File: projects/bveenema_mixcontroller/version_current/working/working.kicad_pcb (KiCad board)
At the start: 2 copper layers, 150.2 x 127 mm, 174 parts, among them J101 B2B-PH-K-S(LF)(SN), J103 B3B-PH-K-S(LF)(SN), J104 B2B-XH-A(LF)(SN), J11 B5B-XH-A(LF)(SN), J13 B8B-XH-A(LF)(SN), J2 B2B-XH-A(LF)(SN), J38 B5B-PH-K-S(LF)(SN), J67 B6B-PH-K-S(LF)(SN), J7 B3B-XH-A(LF)(SN), J9 B2B-XH-A(LF)(SN), J91 B4B-XH-A(LF)(SN), J94 0705430001, J95 B8B-XH-A(LF)(SN), J97 B4B-PH-K-S(LF)(SN), Q1 Q_NMOS_GDS, Q2 Q_NMOS_GDS, U1 Photon, U2 Adafruit_1096, U3 BOB-12009, U4 BOB-12009, U6 HSCDANN005PGAA5, U7 MCP23017_SP, U8 ADS7830

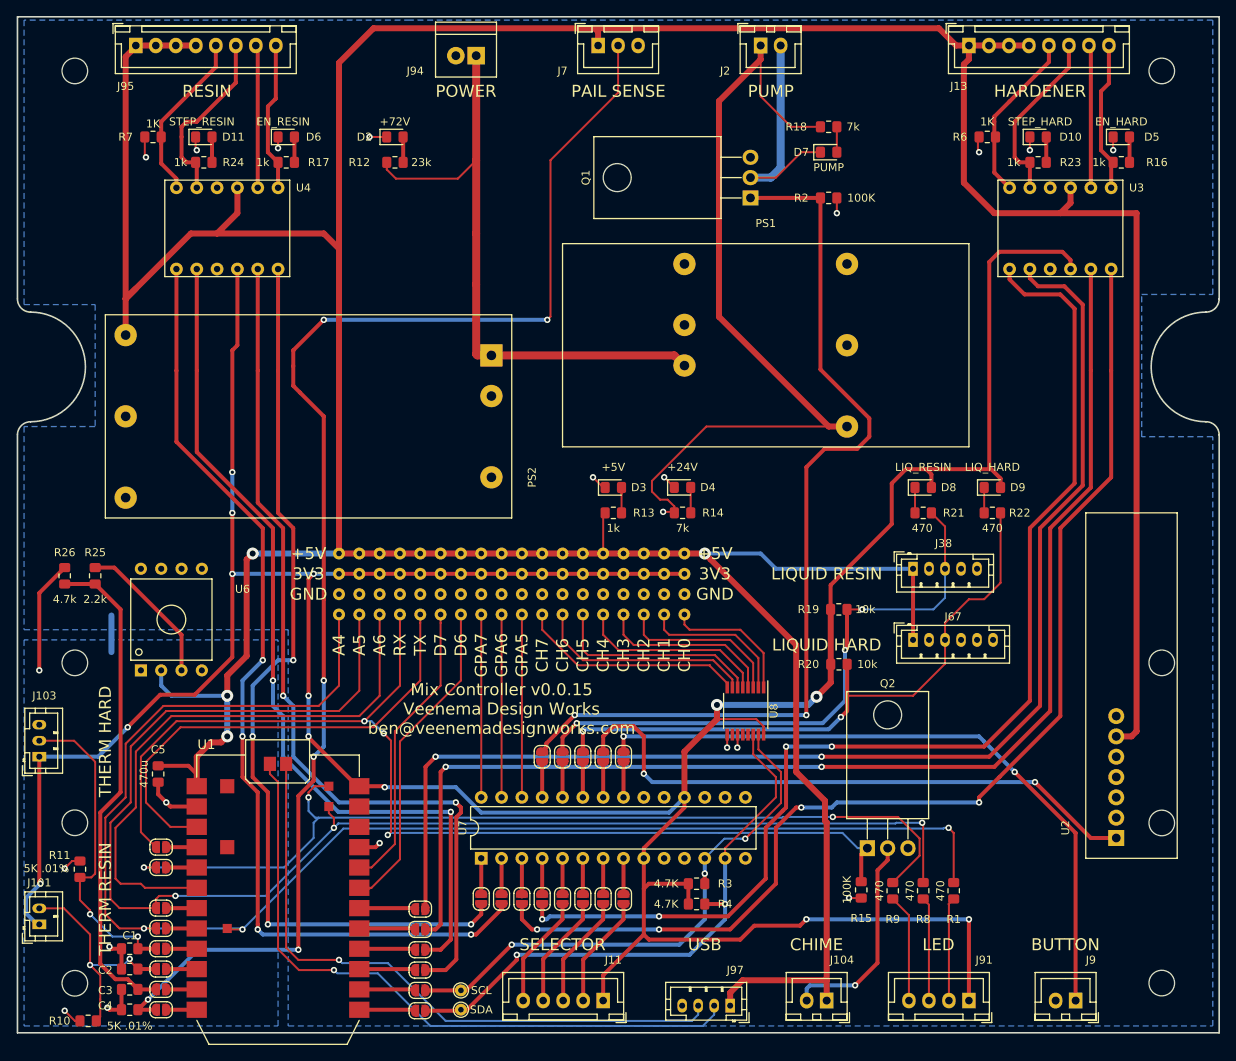
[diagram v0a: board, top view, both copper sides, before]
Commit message: some generations
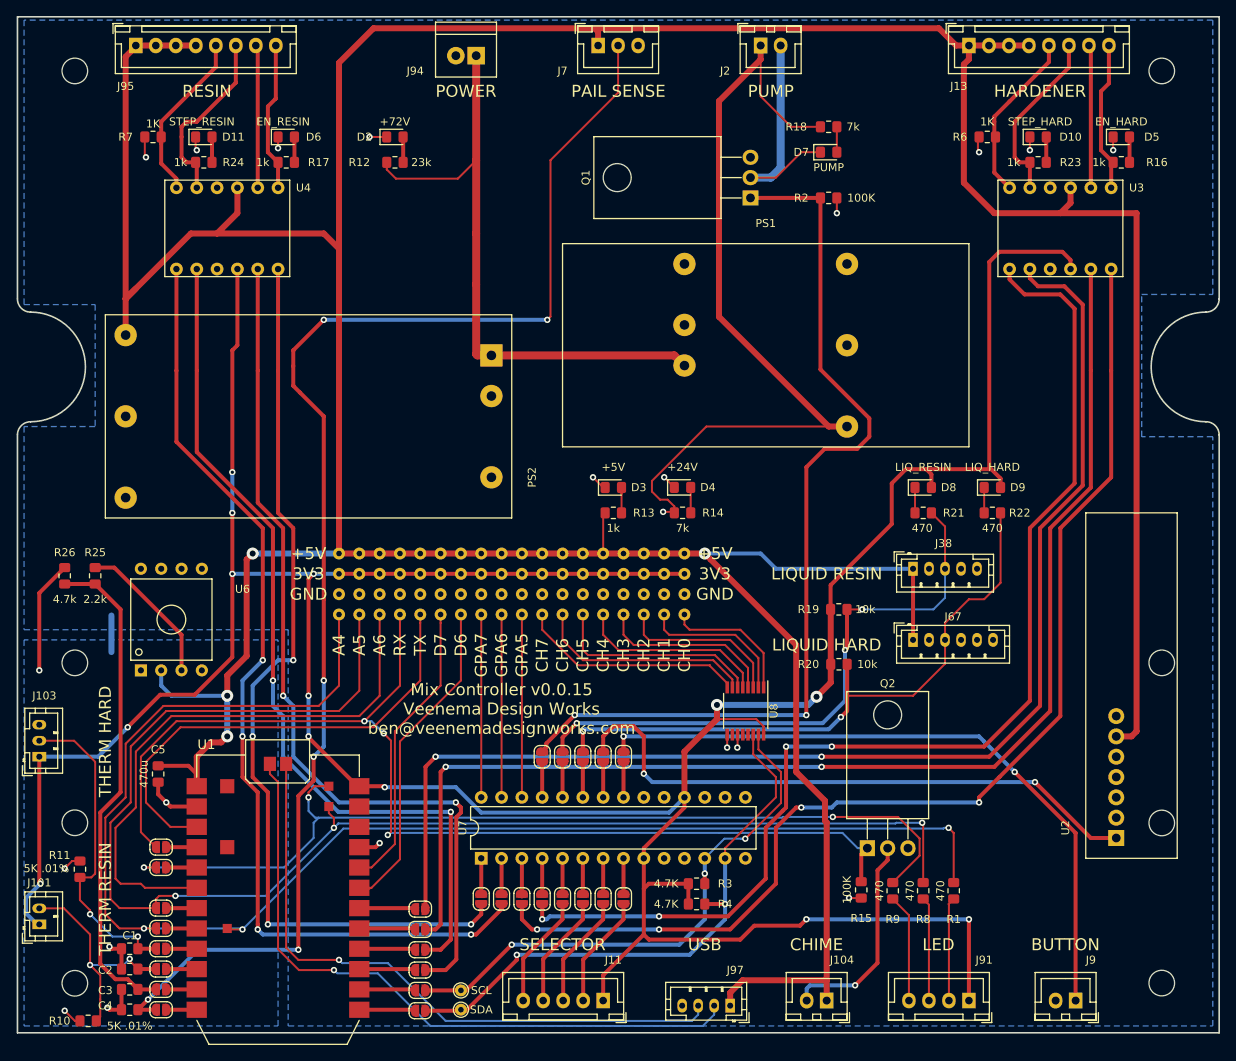
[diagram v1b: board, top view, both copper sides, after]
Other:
- net class Default removed

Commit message: updated all projects from src
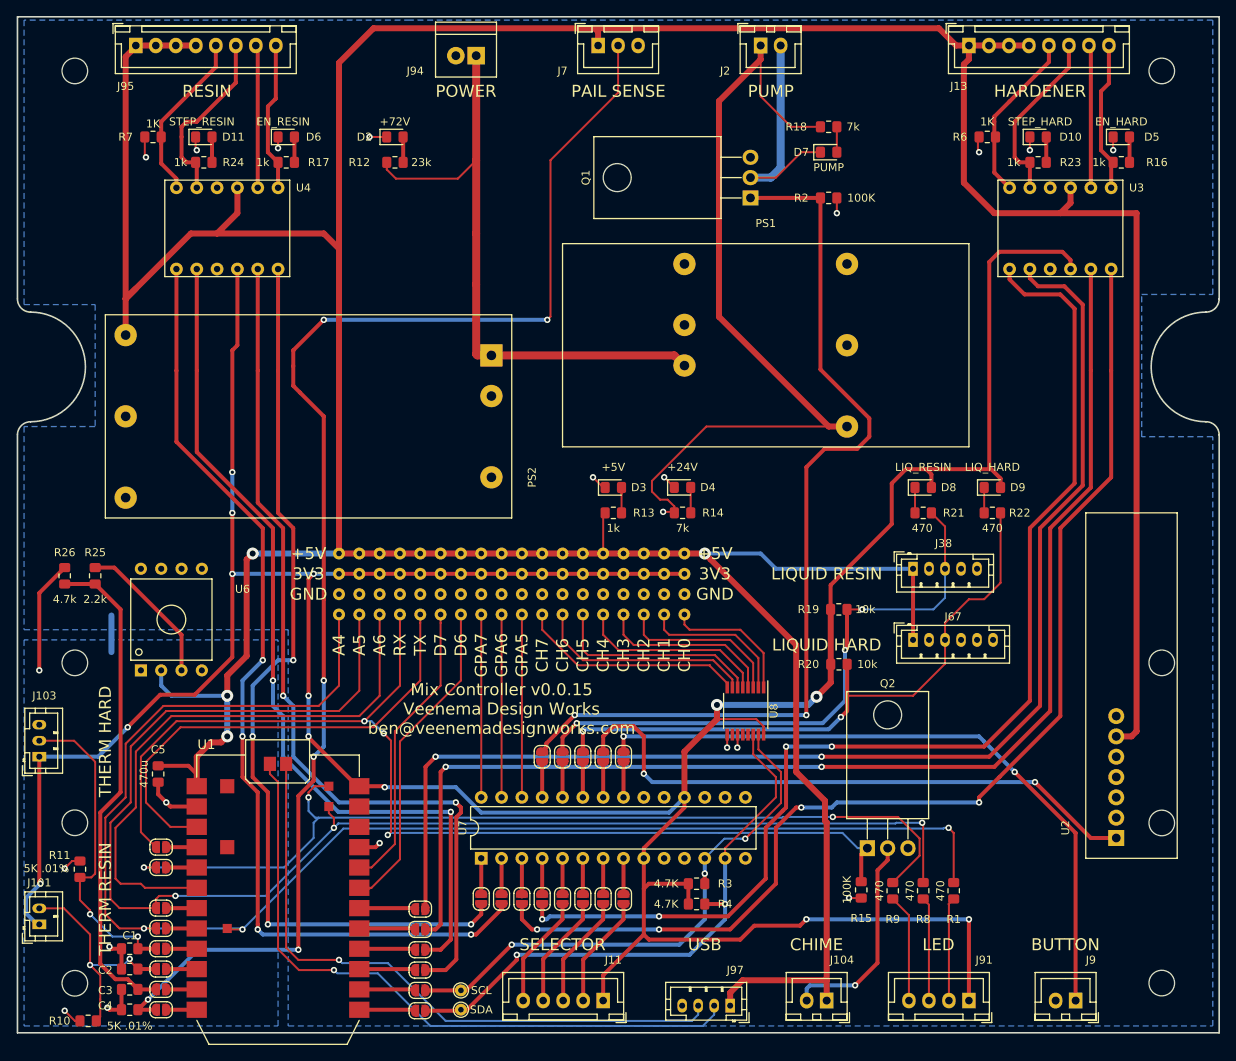
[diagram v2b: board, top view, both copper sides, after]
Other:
- net class Default added: clearance 0.2, trace_width 0.25, via_dia 0.8, via_drill 0.4
